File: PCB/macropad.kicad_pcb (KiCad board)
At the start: 2 copper layers, 64.7 x 84.6 mm, 35 parts, among them J1 Conn_01x04_Socket, SW1 SW_Push, SW10 SW_Push, SW2 SW_Push, SW3 SW_Push, SW4 SW_Push, SW5 SW_Push, SW6 SW_Push, SW7 SW_Push, SW8 SW_Push, SW9 RotaryEncoder_Switch_MP, U1 XIAO-RP2040-DIP

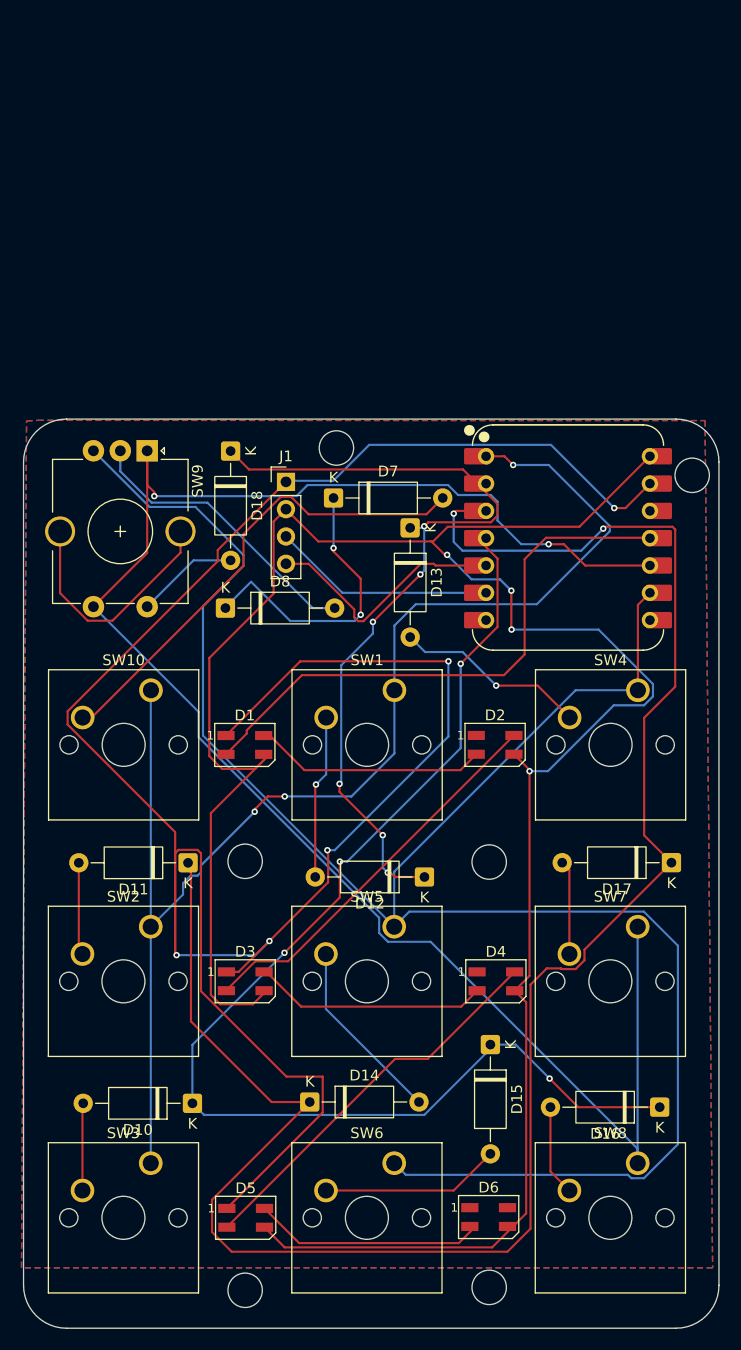
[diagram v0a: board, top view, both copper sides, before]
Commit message: Add files via upload
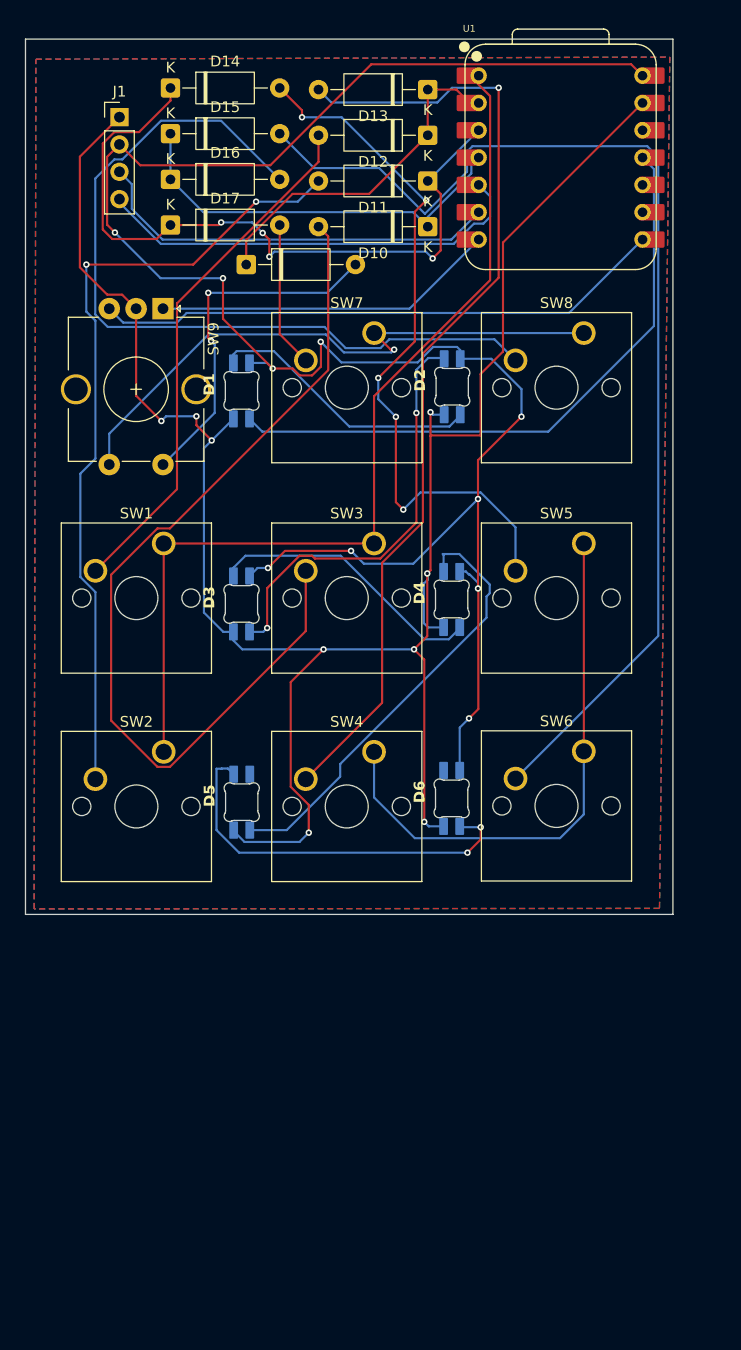
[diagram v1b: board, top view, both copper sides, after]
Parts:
- removed ? (x6): , 
- removed D7, D8: 1N4148WT, Diode_THT:D_A-405_P10.16mm_Horizontal
- removed SW10: SW_Push, Button_Switch_Keyboard:SW_Cherry_MX_1.00u_PCB
- D1, D2, D3, D4, D5, D6: footprint LED_SMD:LED_SK6812MINI_PLCC4_3.5x3.5mm_P1.75mm -> led's:SK6812MINI-E_fixed
- moved D16 97.6 mm to (127.0, 36.9), turned to 0 degrees
- moved D14 95.2 mm to (127.0, 28.4)
- moved D15 89.8 mm to (127.0, 32.7), turned to 0 degrees
- moved D10 84.4 mm to (150.9, 41.3)
- moved SW8 77.4 mm to (165.4, 51.2)
- moved D17 75.4 mm to (127.0, 41.2), turned to 0 degrees
- moved D12 69.0 mm to (150.9, 32.8)
- moved D11 67.2 mm to (150.9, 37.1)
- moved SW3 61.3 mm to (145.9, 70.8)
- moved SW7 60.4 mm to (145.9, 51.2)
- moved SW6 42.2 mm to (165.4, 90.1)
- moved D13 40.8 mm to (150.9, 28.6), turned to 180 degrees
- moved SW5 39.8 mm to (165.4, 70.8)
- moved D6 39.1 mm to (153.2, 94.5), turned to 90 degrees
- moved D5 38.7 mm to (133.7, 94.8), turned to 90 degrees
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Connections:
- SW4 pad 1: col1 -> Net-(SW4-Pad1)
- SW5 pad 1: col1 -> Net-(SW4-Pad1)
- SW6 pad 1: col1 -> Net-(SW4-Pad1)
- SW7 pad 1: col2 -> Net-(SW7-Pad1)
- SW8 pad 1: col2 -> Net-(SW7-Pad1)
- SW9 pad A: col2 -> Net-(U1-GPIO0/TX)
- SW9 pad B: col1 -> Net-(U1-GPIO1/RX)
- SW9 pad C: Net-(D8-A) -> GND
- SW9 pad S2: col2 -> Net-(SW7-Pad1)
- U1 pad 7: unconnected-(U1-GPIO0/TX-Pad7) -> Net-(U1-GPIO0/TX)
- U1 pad 8: unconnected-(U1-GPIO1/RX-Pad8) -> Net-(U1-GPIO1/RX)
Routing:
- net col1: track 180.8 -> 0.00 mm
- net col2: track 169.6 -> 0.00 mm, vias 2 -> 0
- net row1: track 177.4 -> 66.2 mm, vias 2 -> 4
- net Net-(D15-A): track 16.7 -> 105.7 mm
- net Net-(D10-A): track 8.14 -> 86.1 mm
- net row2: track 114.8 -> 38.5 mm, vias 4 -> 0
- net Net-(D13-A): track 17.9 -> 89.5 mm
- net Net-(D16-A): track 8.48 -> 75.8 mm
- net Net-(D11-A): track 8.63 -> 74.2 mm, vias 0 -> 2
- net Net-(SW7-Pad1): track 0.00 -> 56.0 mm, vias 0 -> 1
- net Net-(U1-GPIO1/RX): track 0.00 -> 53.3 mm
- net Net-(SW4-Pad1): track 0.00 -> 51.4 mm
- net Net-(D14-A): track 17.3 -> 66.4 mm, vias 0 -> 5
- net row0: track 77.6 -> 31.9 mm, vias 6 -> 0
- net Net-(D7-A): track 45.0 -> 0.00 mm
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- added copper zone on B.Cu, net +5V
- added copper zone on F.Cu, net +5V
- removed copper zone on B.Cu, net GND
- removed copper zone on F.Cu, net GND
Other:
- board size 64.7 x 84.6 mm -> 60.2 x 81.4 mm
